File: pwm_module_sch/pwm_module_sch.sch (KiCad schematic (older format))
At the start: 48 parts, among them J1 SWIMM, J2 output -, J3 input, J4 output+, J5 uart, Q1 AO3400, Q2 6N60, SW1 ., SW2 ., U1 TM1637, U2 STM8S003F3P, U3 LM358, U4 L78L33

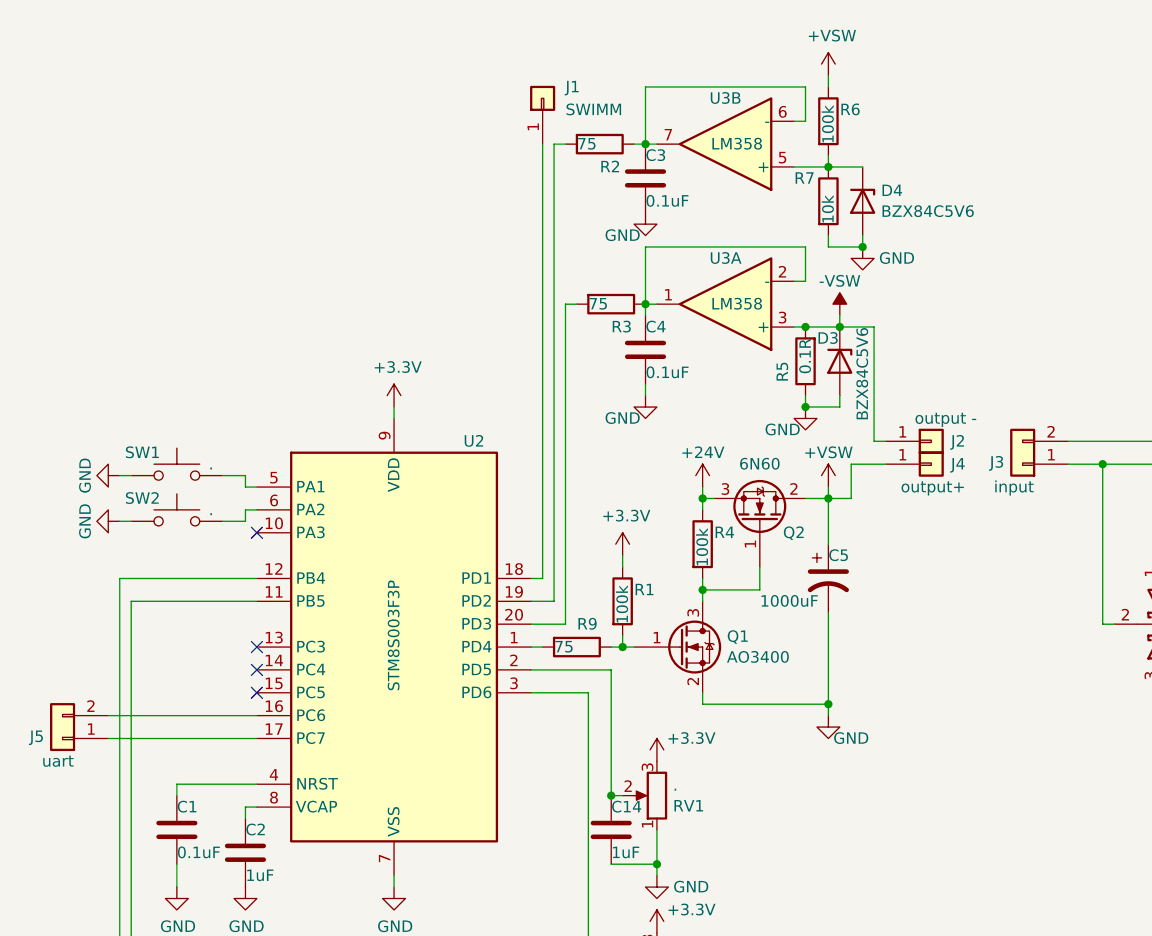
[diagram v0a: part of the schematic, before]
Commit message: reduced dimentions
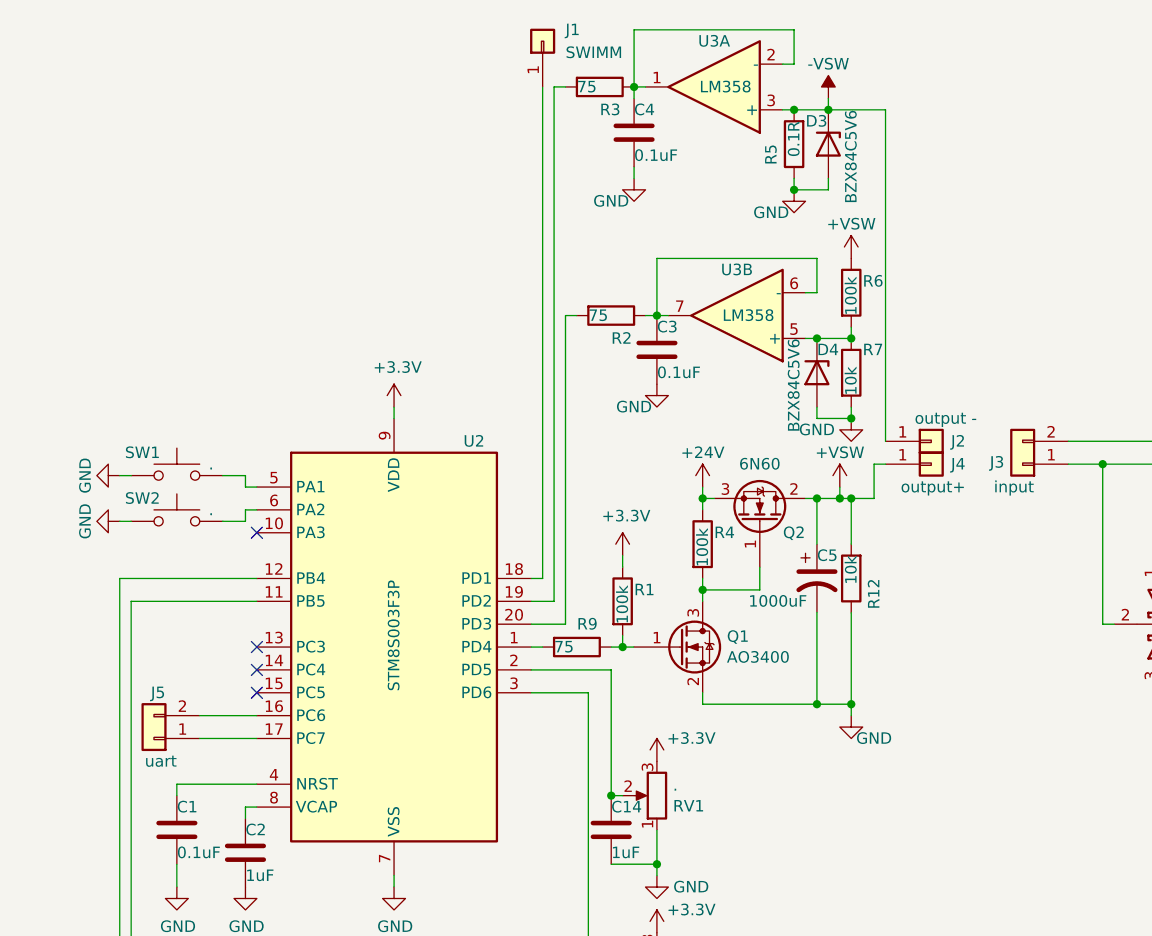
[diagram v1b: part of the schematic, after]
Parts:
- added R12: 10k, Resistor_SMD:R_1210_3225Metric, symbol Device:R
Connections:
- net +VSW: now also R12.2
- net GND: now also R12.1
- net at U2.19 (PD2): now also R3.2; no longer R2.2
- net at U2.20 (PD3): now also R2.2; no longer R3.2
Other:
- moved on the sheet: C3, C4, C5, D3, D4, J1, J5, R2, R3, R5, R6, R7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

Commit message: 0402 caps
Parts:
- C1, C10, C11, C12, C3, C4: footprint Capacitor_SMD:C_0805_2012Metric -> Capacitor_SMD:C_0402_1005Metric
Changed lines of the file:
@@
 F 0 "C1" H 2400 4150 50  0000 L CNN
 F 1 "0.1uF" H 2400 3950 50  0000 L CNN
-F 2 "Capacitor_SMD:C_0805_2012Metric" H 2438 3900 50  0001 C CNN
+F 2 "Capacitor_SMD:C_0402_1005Metric" H 2438 3900 50  0001 C CNN
 F 3 "~" H 2400 4050 50  0001 C CNN
 	1    2400 4050
@@
 F 0 "C10" H 8400 4550 50  0000 L CNN
 F 1 "0.1uF" H 8400 4350 50  0000 L CNN
-F 2 "Capacitor_SMD:C_0805_2012Metric" H 8438 4300 50  0001 C CNN
+F 2 "Capacitor_SMD:C_0402_1005Metric" H 8438 4300 50  0001 C CNN
 F 3 "~" H 8400 4450 50  0001 C CNN
 	1    8400 4450
@@
 F 0 "C11" H 8600 4550 50  0000 L CNN
 F 1 "0.1uF" H 8600 4350 50  0000 L CNN
-F 2 "Capacitor_SMD:C_0805_2012Metric" H 8638 4300 50  0001 C CNN
+F 2 "Capacitor_SMD:C_0402_1005Metric" H 8638 4300 50  0001 C CNN
 F 3 "~" H 8600 4450 50  0001 C CNN
 	1    8600 4450
@@
 F 0 "C12" H 8800 4550 50  0000 L CNN
 F 1 "0.1uF" H 8800 4350 50  0000 L CNN
-F 2 "Capacitor_SMD:C_0805_2012Metric" H 8838 4300 50  0001 C CNN
+F 2 "Capacitor_SMD:C_0402_1005Metric" H 8838 4300 50  0001 C CNN
 F 3 "~" H 8800 4450 50  0001 C CNN
 	1    8800 4450
@@
 F 0 "C4" H 4400 1100 50  0000 L CNN
 F 1 "0.1uF" H 4400 900 50  0000 L CNN
-F 2 "Capacitor_SMD:C_0805_2012Metric" H 4438 850 50  0001 C CNN
+F 2 "Capacitor_SMD:C_0402_1005Metric" H 4438 850 50  0001 C CNN
 F 3 "~" H 4400 1000 50  0001 C CNN
 	1    4400 1000
@@
 F 0 "C3" H 4500 2050 50  0000 L CNN
 F 1 "0.1uF" H 4500 1850 50  0000 L CNN
-F 2 "Capacitor_SMD:C_0805_2012Metric" H 4538 1800 50  0001 C CNN
+F 2 "Capacitor_SMD:C_0402_1005Metric" H 4538 1800 50  0001 C CNN
 F 3 "~" H 4500 1950 50  0001 C CNN
 	1    4500 1950
